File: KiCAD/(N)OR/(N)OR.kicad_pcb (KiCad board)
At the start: 2 copper layers, 71.1 x 62.2 mm, 18 parts, among them J1 Conn_01x02_Pin, J2 Conn_01x02_Pin, J3 Conn_01x02_Pin, J4 Conn_01x02_Pin, Q13 2N7000, Q14 2N7000, Q15 2N7000, Q3 2N7000, Q4 2N7000, Q5 2N7000, Y1 Conn_01x01_Pin, Y2 Conn_01x01_Pin

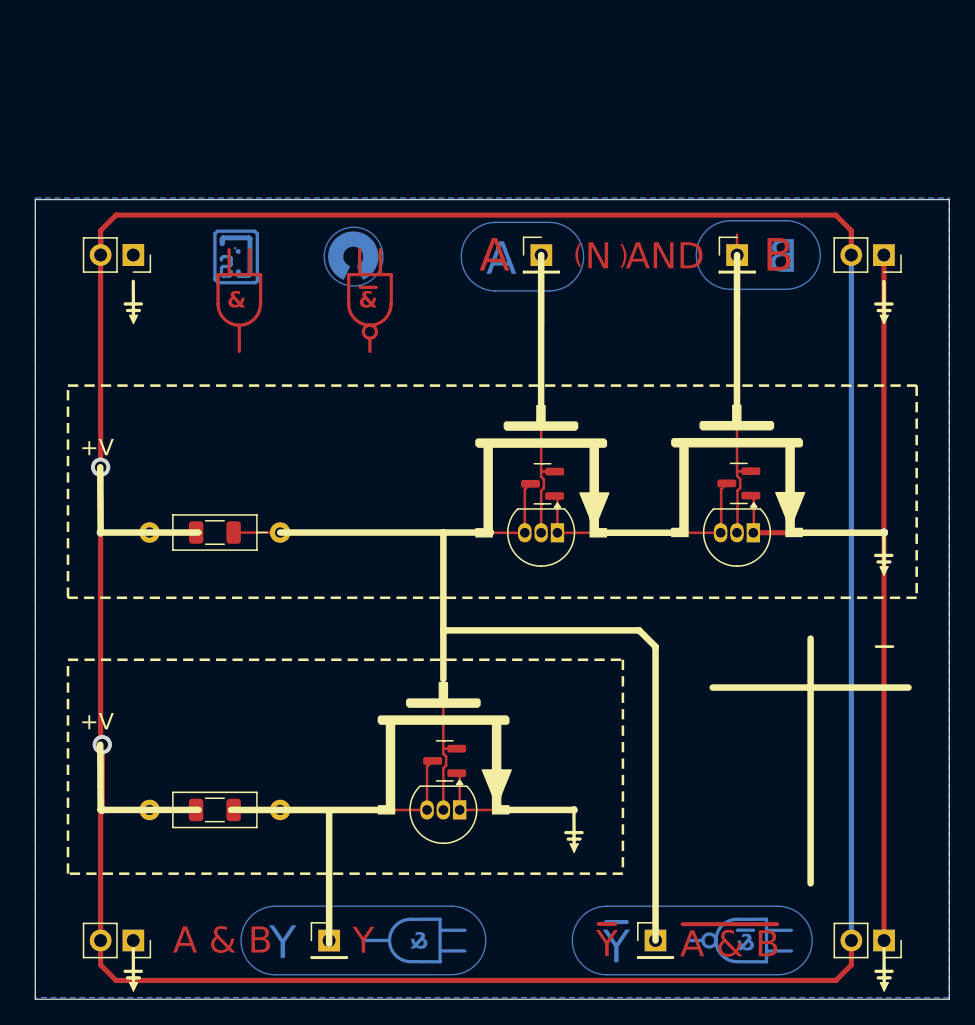
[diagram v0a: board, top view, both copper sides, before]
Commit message: (N)OR
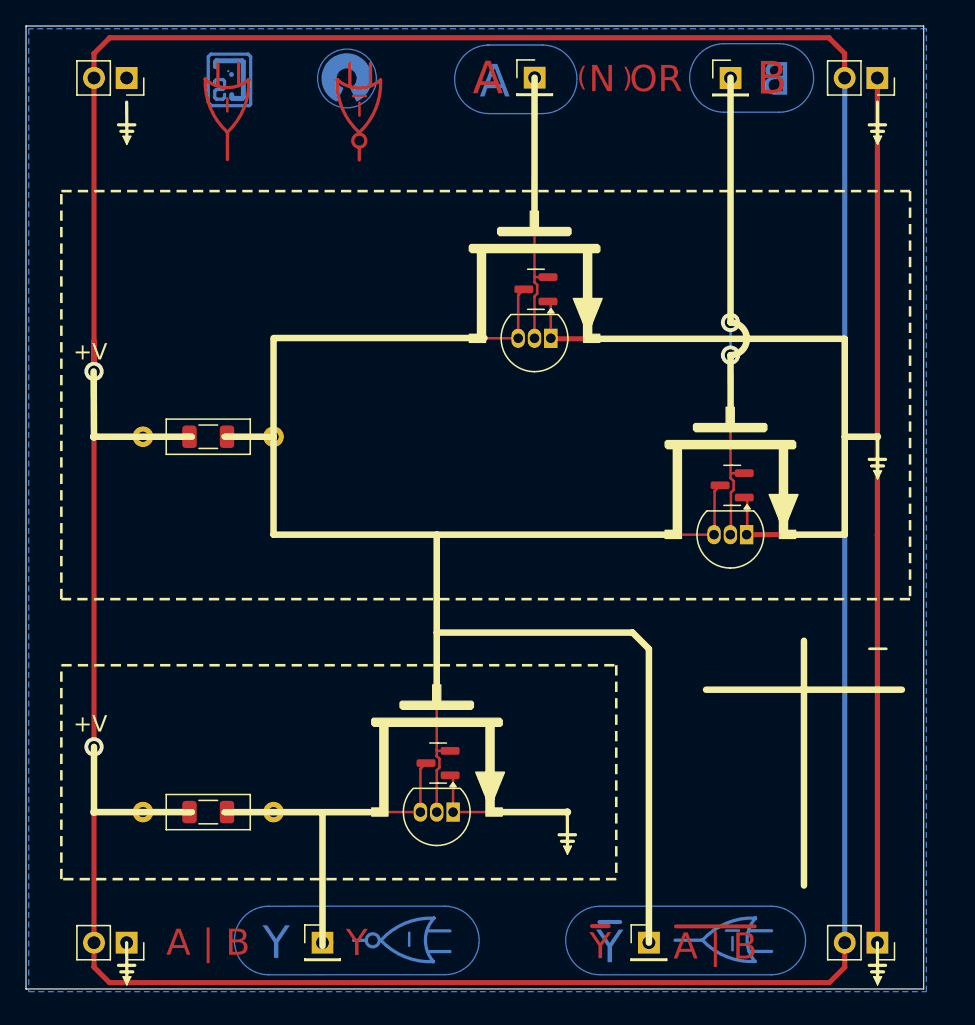
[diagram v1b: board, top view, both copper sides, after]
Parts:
- moved Q3 15.1 mm to (234.9, 101.6)
- moved Q13 15.1 mm to (233.8, 97.8)
- moved A1 13.8 mm to (233.7, 81.3)
- moved B1 13.8 mm to (248.9, 81.3)
- moved J4 13.8 mm to (260.3, 81.3)
- moved J1 13.8 mm to (201.9, 81.3)
- moved R15 7.47 mm to (208.3, 109.3)
- moved R5 7.47 mm to (203.2, 109.3)
- moved J2 0.54 mm to (201.9, 148.6)
- moved J3 0.54 mm to (260.3, 148.6)
- moved Q15 0.54 mm to (226.2, 134.7)
- moved Q5 0.54 mm to (227.3, 138.5)
- moved R16 0.54 mm to (208.3, 138.5)
- moved R6 0.54 mm to (203.2, 138.5)
- moved Y2 0.54 mm to (242.6, 148.6)
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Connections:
- Q13 pad 1: Net-(Q13-S) -> GNDREF
- Q14 pad 3: Net-(Q13-S) -> Net-(Q13-D)
- Q3 pad 1: Net-(Q13-S) -> GNDREF
- Q4 pad 3: Net-(Q13-S) -> Net-(Q13-D)
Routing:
- net GNDREF: track 78.3 -> 133.1 mm, vias 5 -> 2
- net Net-(Q13-D): track 89.3 -> 142.9 mm
- net VDD: track 263.6 -> 287.1 mm, vias 6 -> 5
- net Net-(Q13-S): track 19.6 -> 0.00 mm
- net Net-(B1-Pin_1): track 24.4 -> 36.7 mm, vias 0 -> 2
- net (no net): track 48.6 -> 38.9 mm
- net Net-(A1-Pin_1): track 27.9 -> 25.1 mm
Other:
- board size 71.1 x 62.2 mm -> 69.8 x 74.9 mm
- board text added: "1st Digit"
- board text added: "2nd Digit"
- board text added: "A | B"
- board text added: "Number"
- board text added: "OR"
- board text added: "Resistor Colour Code"
- board text added: "of 0's"
- board text added: "~{A | B}"
- board text removed: "&"
- board text removed: "+V Opens the Gate"
- board text removed: "A & B"
- board text removed: "AND"
- board text removed: "DRAIN"
- board text removed: "Drains power from +V"
- board text removed: "GATE"
- board text removed: "MOSFET"
- board text removed: "N-Channel"
- board text removed: "N-Channel MOSFET :"
- board text removed: "Provides a power Source"
- board text removed: "SOURCE"
- board text removed: "~{&}"
- board text removed: "~{A & B}"
